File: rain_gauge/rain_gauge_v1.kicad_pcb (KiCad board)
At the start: 2 copper layers, 30 x 30 mm, 20 parts, among them J1 Conn_01x05_Pin, SW1 SW_Reed, U1 S35770, U2 SN74LVC1G14DBV, U3 AP2112K-3.3

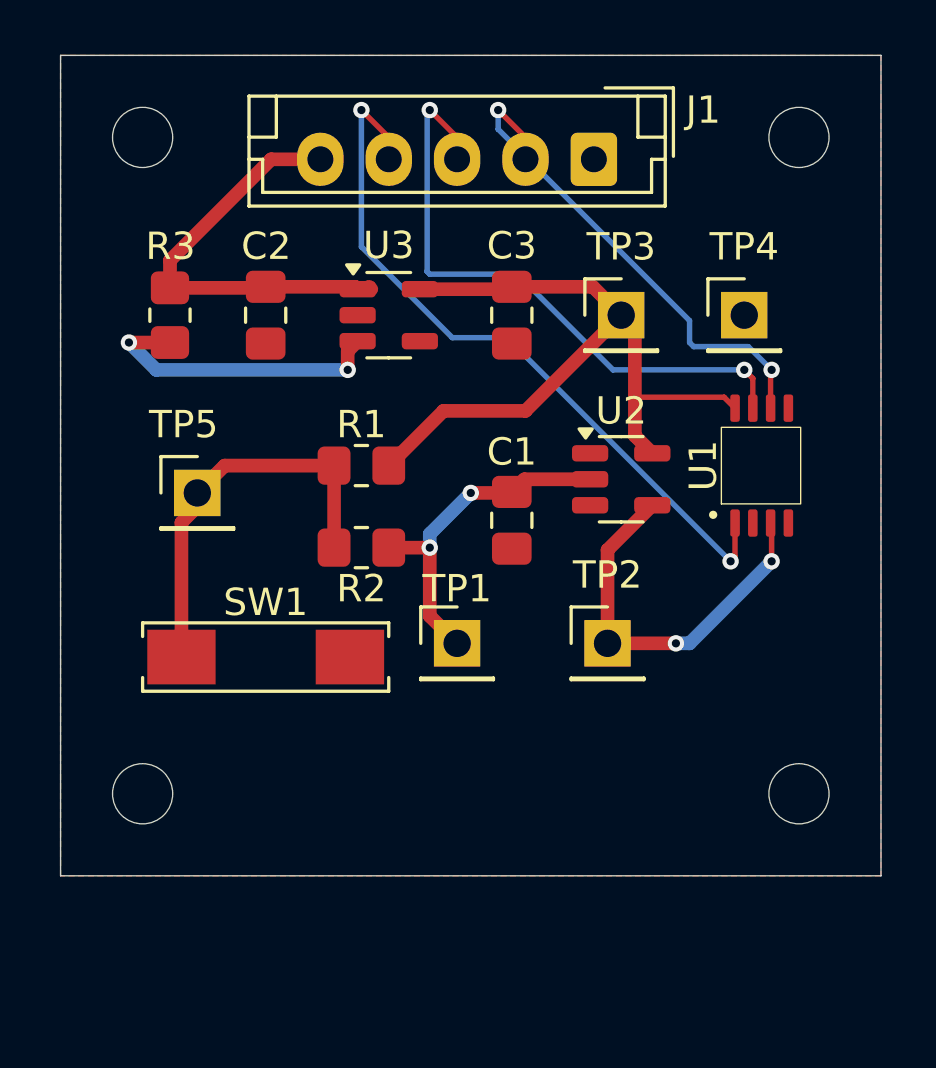
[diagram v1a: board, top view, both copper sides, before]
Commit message: Rain Gauge V2
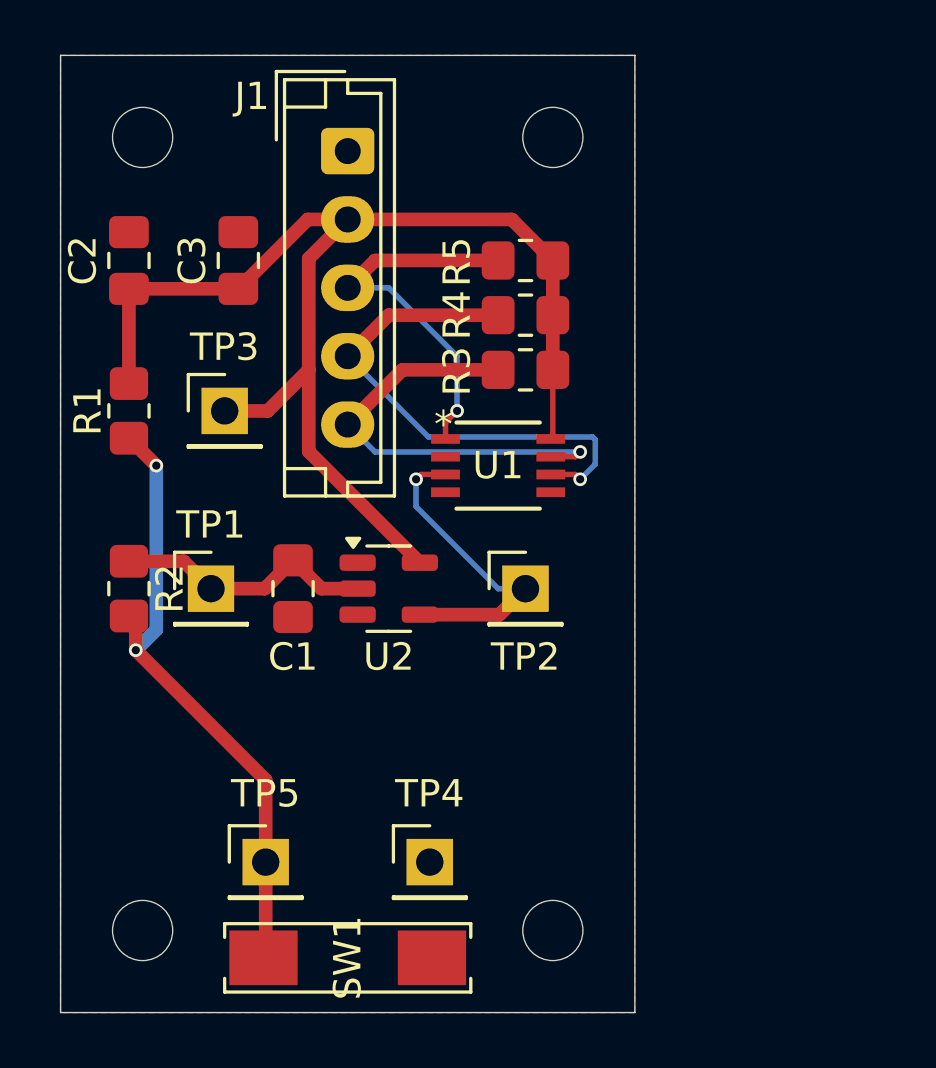
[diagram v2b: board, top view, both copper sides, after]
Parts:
- removed U3: AP2112K-3.3, Package_TO_SOT_SMD:SOT-23-5
- added R4: 1K DNF, Resistor_SMD:R_0805_2012Metric_Pad1.20x1.40mm_HandSolder, F.Cu at (130.0, 96.5)
- added R5: 10K DNF, Resistor_SMD:R_0805_2012Metric_Pad1.20x1.40mm_HandSolder, F.Cu at (130.0, 94.5)
- R3: value R -> 1K DNF
- U1: footprint Package_TMSOP:TMSOP8 -> WiSDOM:TMSOP08_2P9X2P8_ABL
- moved TP4 23.1 mm to (126.5, 116.5)
- moved TP3 14.9 mm to (119.0, 100.0)
- moved TP5 13.7 mm to (120.5, 116.5)
- moved R3 13.2 mm to (130.0, 98.5), turned to 180 degrees
- moved SW1 11.4 mm to (123.5, 120.0)
- moved REF** 10.3 mm to (131.0, 119.0)
- moved C3 10.2 mm to (119.5, 94.5), turned to 90 degrees
- moved U2 9.39 mm to (125.0, 106.5)
- moved TP1 9.22 mm to (118.5, 106.5)
- moved J1 9.00 mm to (123.5, 90.5), turned to -90 degrees
- moved REF** 9.00 mm to (131.0, 90.0)
- moved R1 8.73 mm to (115.5, 100.0), turned to -90 degrees
- moved R2 8.63 mm to (115.5, 106.5), turned to 90 degrees
- moved C1 8.38 mm to (121.5, 106.5)
- moved C2 5.39 mm to (115.5, 94.5), turned to 90 degrees
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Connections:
- C2 pad 1: VCC -> +3.3V
- C3 pad 1: VREG -> +3.3V
- J1 pad 2: SDA -> +3.3V
- J1 pad 3: SCL -> ~RST
- J1 pad 4: ~RST -> SDA
- J1 pad 5: VCC -> SCL
- R1 pad 1: VREG -> +3.3V
- R3 pad 1: VCC -> +3.3V
- R3 pad 2: Net-(U3-EN) -> SCL
- TP3 pad 1: VREG -> +3.3V
- U1 pad 8: VREG -> +3.3V
- U2 pad 5: VREG -> +3.3V
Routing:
- net +3.3V: track 0.00 -> 45.7 mm
- net VREG: track 28.0 -> 0.00 mm
- net VCC: track 15.1 -> 0.00 mm
- net ~RST: track 27.6 -> 14.2 mm, vias 2 -> 1
- net Net-(U3-EN): track 11.1 -> 0.00 mm, vias 2 -> 0
- net Net-(R1-Pad2): track 14.2 -> 23.1 mm, vias 0 -> 2
- net SCL: track 22.8 -> 16.4 mm, vias 2 -> 1
- net Net-(C1-Pad1): track 12.7 -> 9.64 mm, vias 2 -> 0
- net CLKIN: track 14.4 -> 11.6 mm, vias 2 -> 1
- net SDA: track 18.4 -> 19.3 mm, vias 2 -> 1
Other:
- board size 30 x 30 mm -> 21 x 35 mm
